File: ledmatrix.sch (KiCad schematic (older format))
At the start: 58 parts, among them P3 CONN_01X12, U58 sled1735

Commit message: led fp
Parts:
- removed P3: CONN_01X12, fp:FPC_12, symbol CONN_01X12
- removed rgb-i5, rgb-j5, rgb-k5, rgb-l5, rgb-o5, rgb-p5: rgbled, fp:WL-SFRW-REV, symbol rgbled
- added P3: CONN_01X10, fp:FPC_10, symbol CONN_01X10
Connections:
- net labels added: ca9, cb1, cb2, cb4, cb5, cb6
- wire segments 47 -> 53
- no-connect marks 7 -> 5
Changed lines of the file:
@@
 $EndComp
 $Comp
-L Earth #PWR035
+L Earth #PWR037
 U 1 1 59AF6699
 P 9050 2250
-F 0 "#PWR035" H 9050 2000 50  0001 C CNN
+F 0 "#PWR037" H 9050 2000 50  0001 C CNN
 F 1 "Earth" H 9050 2100 50  0001 C CNN
 F 2 "" H 9050 2250 50  0000 C CNN
@@
 $EndComp
 $Comp
-L Earth #PWR036
+L Earth #PWR038
 U 1 1 59AF6F30
 P 9500 4250
-F 0 "#PWR036" H 9500 4000 50  0001 C CNN
+F 0 "#PWR038" H 9500 4000 50  0001 C CNN
 F 1 "Earth" H 9500 4100 50  0001 C CNN
 F 2 "" H 9500 4250 50  0000 C CNN
@@
 SHUTDOWN
 $Comp
-L +5V #PWR037
+L +5V #PWR039
 U 1 1 59AFE176
 P 9050 1950
-F 0 "#PWR037" H 9050 1800 50  0001 C CNN
+F 0 "#PWR039" H 9050 1800 50  0001 C CNN
 F 1 "+5V" H 9065 2123 50  0000 C CNN
 F 2 "" H 9050 1950 50  0000 C CNN
@@
 	11000 2950 10600 2950
 NoConn ~ 11000 3050
-$Comp
-L CONN_01X12 P3
-U 1 1 59D3F06A
-P 11200 2700
-F 0 "P3" H 11278 2741 50  0000 L CNN
-F 1 "CONN_01X12" H 11278 2650 50  0000 L CNN
-F 2 "fp:FPC_12" H 11200 2700 50  0001 C CNN
-F 3 "" H 11200 2700 50  0000 C CNN
-F 4 "2458999" H 11200 2700 60  0001 C CNN "farnell #"
-	1    11200 2700
-	1    0    0    -1
-$EndComp
-NoConn ~ 11000 3150
-NoConn ~ 11000 3250
 Text Notes 2200 300  0    197  ~ 0
 common anode type 3 matrix
-$Comp
-L rgbled rgb-i5
-U 1 1 59D7718B
-P 4750 5100
-F 0 "rgb-i5" H 4581 5239 60  0000 R CNN
-F 1 "rgbled" H 4581 5133 60  0000 R CNN
-F 2 "fp:WL-SFRW-REV" H 4750 5100 60  0001 C CNN
-F 3 "" H 4750 5100 60  0001 C CNN
-	1    4750 5100
-	-1   0    0    -1
-$EndComp
-$Comp
-L rgbled rgb-j5
-U 1 1 59D77215
-P 5150 5100
-F 0 "rgb-j5" H 4981 5239 60  0000 R CNN
-F 1 "rgbled" H 4981 5133 60  0000 R CNN
-F 2 "fp:WL-SFRW-REV" H 5150 5100 60  0001 C CNN
-F 3 "" H 5150 5100 60  0001 C CNN
-	1    5150 5100
-	-1   0    0    -1
-$EndComp
-$Comp
-L rgbled rgb-k5
-U 1 1 59D7729D
-P 5550 5100
-F 0 "rgb-k5" H 5381 5239 60  0000 R CNN
-F 1 "rgbled" H 5381 5133 60  0000 R CNN
-F 2 "fp:WL-SFRW-REV" H 5550 5100 60  0001 C CNN
-F 3 "" H 5550 5100 60  0001 C CNN
-	1    5550 5100
-	-1   0    0    -1
-$EndComp
-$Comp
-L rgbled rgb-l5
-U 1 1 59D77327
-P 5950 5100
-F 0 "rgb-l5" H 5781 5239 60  0000 R CNN
-F 1 "rgbled" H 5781 5133 60  0000 R CNN
-F 2 "fp:WL-SFRW-REV" H 5950 5100 60  0001 C CNN
-F 3 "" H 5950 5100 60  0001 C CNN
-	1    5950 5100
-	-1   0    0    -1
-$EndComp
-$Comp
-L rgbled rgb-o5
-U 1 1 59D77493
-P 7150 5100
-F 0 "rgb-o5" H 6981 5239 60  0000 R CNN
-F 1 "rgbled" H 6981 5133 60  0000 R CNN
-F 2 "fp:WL-SFRW-REV" H 7150 5100 60  0001 C CNN
-F 3 "" H 7150 5100 60  0001 C CNN
-	1    7150 5100
-	-1   0    0    -1
-$EndComp
-$Comp
-L rgbled rgb-p5
-U 1 1 59D775AF
-P 7550 5100
-F 0 "rgb-p5" H 7381 5239 60  0000 R CNN
-F 1 "rgbled" H 7381 5133 60  0000 R CNN
-F 2 "fp:WL-SFRW-REV" H 7550 5100 60  0001 C CNN
-F 3 "" H 7550 5100 60  0001 C CNN
-	1    7550 5100
-	-1   0    0    -1
-$EndComp
 Connection ~ 6950 4800
 Connection ~ 6950 5100
+Text GLabel 3850 6200 0    60   Input ~ 0
+cb4
+Text GLabel 3850 6300 0    60   Input ~ 0
+cb5
+Text GLabel 3850 6400 0    60   Input ~ 0
+cb6
+Text GLabel 3850 6650 0    60   Input ~ 0
+ca9
+Text GLabel 3850 6750 0    60   Input ~ 0
+cb1
+Text GLabel 3850 6850 0    60   Input ~ 0
+cb2
+Text Label 4400 6750 2    60   ~ 0
+CB1
+Text Label 4400 6850 2    60   ~ 0
+CB2
+Text Label 4400 6200 2    60   ~ 0
+CB4
+Text Label 4400 6300 2    60   ~ 0
+CB5
+Text Label 4400 6400 2    60   ~ 0
+CB6
+Text Label 4400 6650 2    60   ~ 0
+CA9
+Wire Wire Line
+	3850 6200 4400 6200
+Wire Wire Line
+	4400 6300 3850 6300
+Wire Wire Line
+	4400 6400 3850 6400
+Wire Wire Line
+	4400 6650 3850 6650
+Wire Wire Line
+	4400 6850 3850 6850
+Wire Wire Line
+	4400 6750 3850 6750
+$Comp
+L CONN_01X10 P3
+U 1 1 59D903C8
+P 11200 2600
+F 0 "P3" H 11278 2641 50  0000 L CNN
+F 1 "CONN_01X10" H 11278 2550 50  0000 L CNN
+F 2 "fp:FPC_10" H 11200 2600 50  0001 C CNN
+F 3 "" H 11200 2600 50  0000 C CNN
+	1    11200 2600
+	1    0    0    -1
+$EndComp
 $EndSCHEMATC

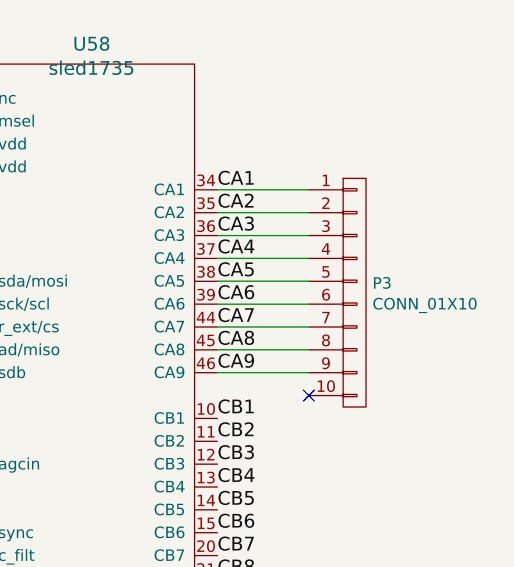
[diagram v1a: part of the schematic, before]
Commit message: routing
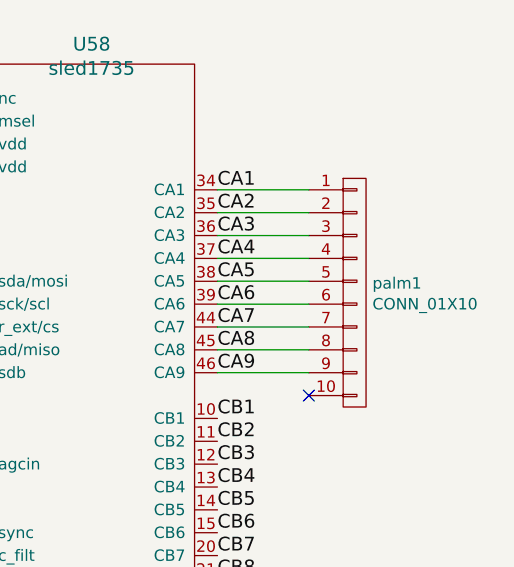
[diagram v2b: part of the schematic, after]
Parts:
- renumbered P3 to palm1
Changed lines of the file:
@@
 	4400 6750 3850 6750
 $Comp
-L CONN_01X10 P3
+L CONN_01X10 palm1
 U 1 1 59D903C8
 P 11200 2600
-F 0 "P3" H 11278 2641 50  0000 L CNN
+F 0 "palm1" H 11278 2641 50  0000 L CNN
 F 1 "CONN_01X10" H 11278 2550 50  0000 L CNN
 F 2 "fp:FPC_10" H 11200 2600 50  0001 C CNN

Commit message: fab with 0.16 clearance
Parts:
- U58: footprint fp:QFN-56_EP_4.5x6.5_Pitch0.4mm -> fp:QFN-56_EP_4.5x6.5_Pitch0.4mm_fanout
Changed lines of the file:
@@
 F 0 "U58" H 10050 2987 60  0000 C CNN
 F 1 "sled1735" H 10050 2881 60  0000 C CNN
-F 2 "fp:QFN-56_EP_4.5x6.5_Pitch0.4mm" H 9850 2250 60  0001 C CNN
+F 2 "fp:QFN-56_EP_4.5x6.5_Pitch0.4mm_fanout" H 9850 2250 60  0001 C CNN
 F 3 "" H 9850 2250 60  0001 C CNN
 	1    9850 2250
@@
 $EndComp
 $Comp
-L Earth #PWR037
+L Earth #PWR031
 U 1 1 59AF6699
 P 9050 2250
-F 0 "#PWR037" H 9050 2000 50  0001 C CNN
+F 0 "#PWR031" H 9050 2000 50  0001 C CNN
 F 1 "Earth" H 9050 2100 50  0001 C CNN
 F 2 "" H 9050 2250 50  0000 C CNN
@@
 $EndComp
 $Comp
-L Earth #PWR038
+L Earth #PWR032
 U 1 1 59AF6F30
 P 9500 4250
-F 0 "#PWR038" H 9500 4000 50  0001 C CNN
+F 0 "#PWR032" H 9500 4000 50  0001 C CNN
 F 1 "Earth" H 9500 4100 50  0001 C CNN
 F 2 "" H 9500 4250 50  0000 C CNN
@@
 SHUTDOWN
 $Comp
-L +5V #PWR039
+L +5V #PWR033
 U 1 1 59AFE176
 P 9050 1950
-F 0 "#PWR039" H 9050 1800 50  0001 C CNN
+F 0 "#PWR033" H 9050 1800 50  0001 C CNN
 F 1 "+5V" H 9065 2123 50  0000 C CNN
 F 2 "" H 9050 1950 50  0000 C CNN

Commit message: component order codes
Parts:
- C6: farnell # 1759454 -> 1759422
- C7: farnell # 1414715 -> 1759167
- U58: footprint fp:QFN-56_EP_4.5x6.5_Pitch0.4mm_fanout -> fp:QFN-56_EP_4.5x6.5_Pitch0.4mm
- palm1: farnell # (none) -> 1302345
- rgb-h1: farnell # (none) -> 2765007
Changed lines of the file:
@@
 F 2 "fp:WL-SFRW-REV" H 4350 1500 60  0001 C CNN
 F 3 "" H 4350 1500 60  0001 C CNN
+F 4 "2765007" H 4350 1500 60  0001 C CNN "farnell #"
 	1    4350 1500
 	1    0    0    -1
@@
 F 0 "U58" H 10050 2987 60  0000 C CNN
 F 1 "sled1735" H 10050 2881 60  0000 C CNN
-F 2 "fp:QFN-56_EP_4.5x6.5_Pitch0.4mm_fanout" H 9850 2250 60  0001 C CNN
+F 2 "fp:QFN-56_EP_4.5x6.5_Pitch0.4mm" H 9850 2250 60  0001 C CNN
 F 3 "" H 9850 2250 60  0001 C CNN
 	1    9850 2250
@@
 F 2 "Capacitors_SMD:C_0805" H 9088 1950 50  0001 C CNN
 F 3 "" H 9050 2100 50  0000 C CNN
-F 4 "1414715" H 9050 2100 60  0001 C CNN "farnell #"
+F 4 "1759167" H 9050 2100 60  0001 C CNN "farnell #"
 	1    9050 2100
 	1    0    0    -1
@@
 F 2 "Capacitors_SMD:C_0805" H 8738 1950 50  0001 C CNN
 F 3 "" H 8700 2100 50  0000 C CNN
-F 4 "1759454" H 8700 2100 60  0001 C CNN "farnell #"
+F 4 "1759422" H 8700 2100 60  0001 C CNN "farnell #"
 	1    8700 2100
 	1    0    0    -1
@@
 F 2 "fp:FPC_10" H 11200 2600 50  0001 C CNN
 F 3 "" H 11200 2600 50  0000 C CNN
+F 4 "1302345" H 11200 2600 60  0001 C CNN "farnell #"
 	1    11200 2600
 	1    0    0    -1
